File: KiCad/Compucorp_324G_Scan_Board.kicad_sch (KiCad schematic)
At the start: 14 parts, among them J1 BR 16252, J2 Power In, J4 From Keyboard, U1 BR 16252

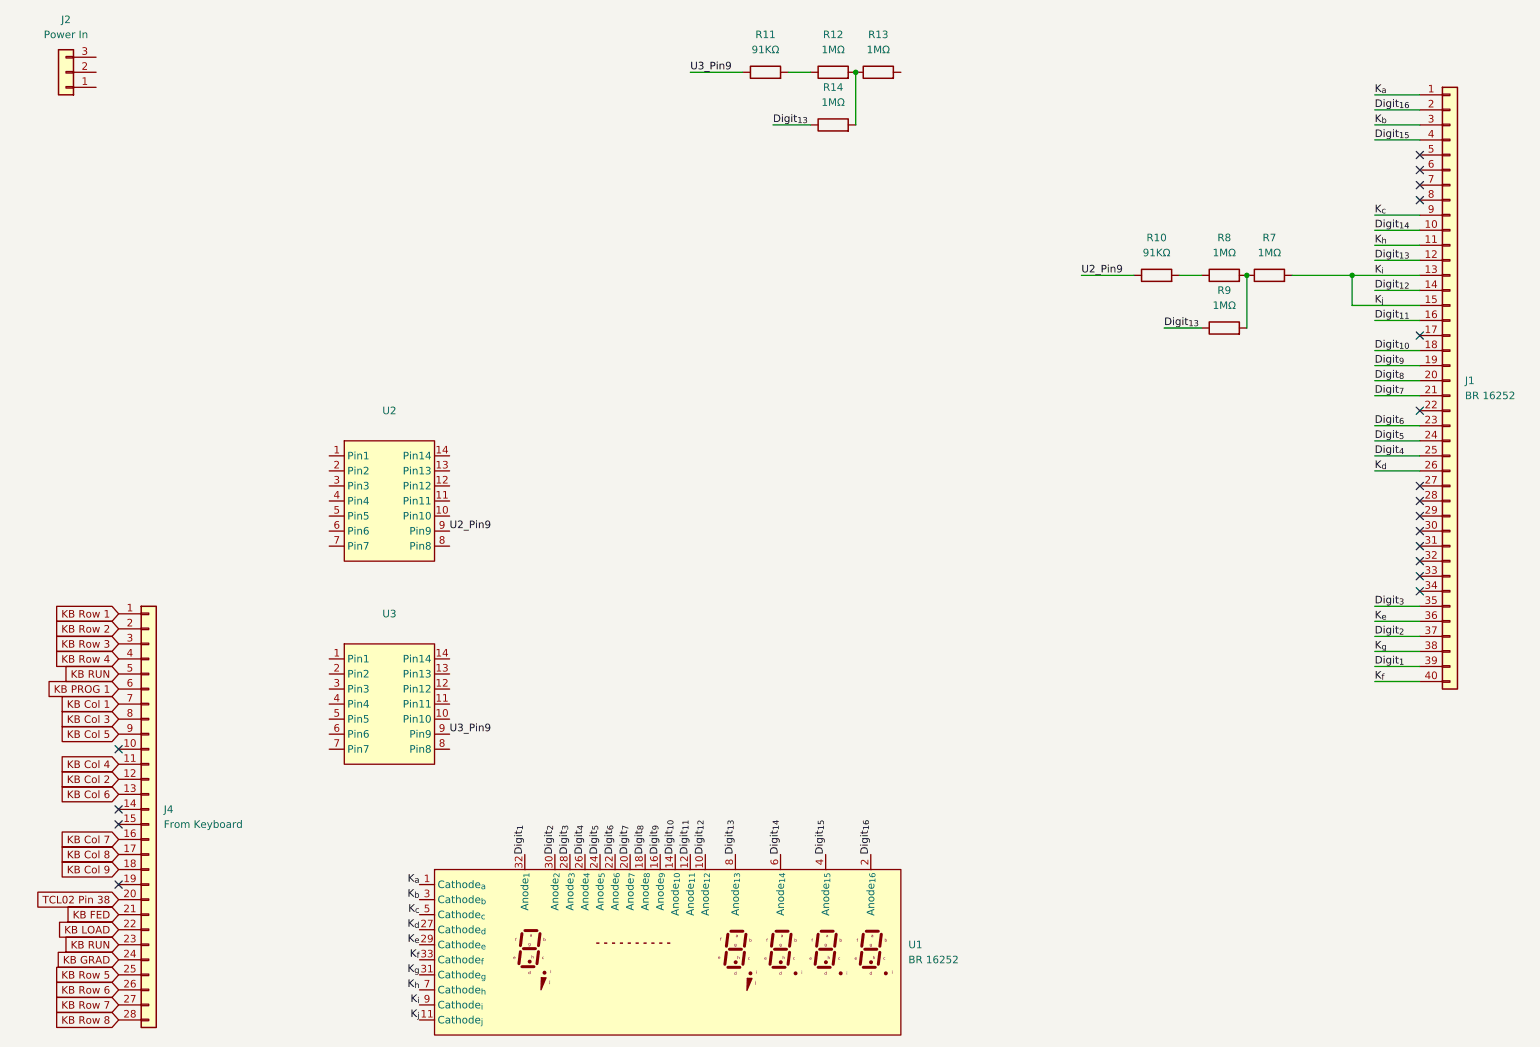
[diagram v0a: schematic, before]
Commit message: Update Compucorp_324G_Scan_Board.kicad_sch
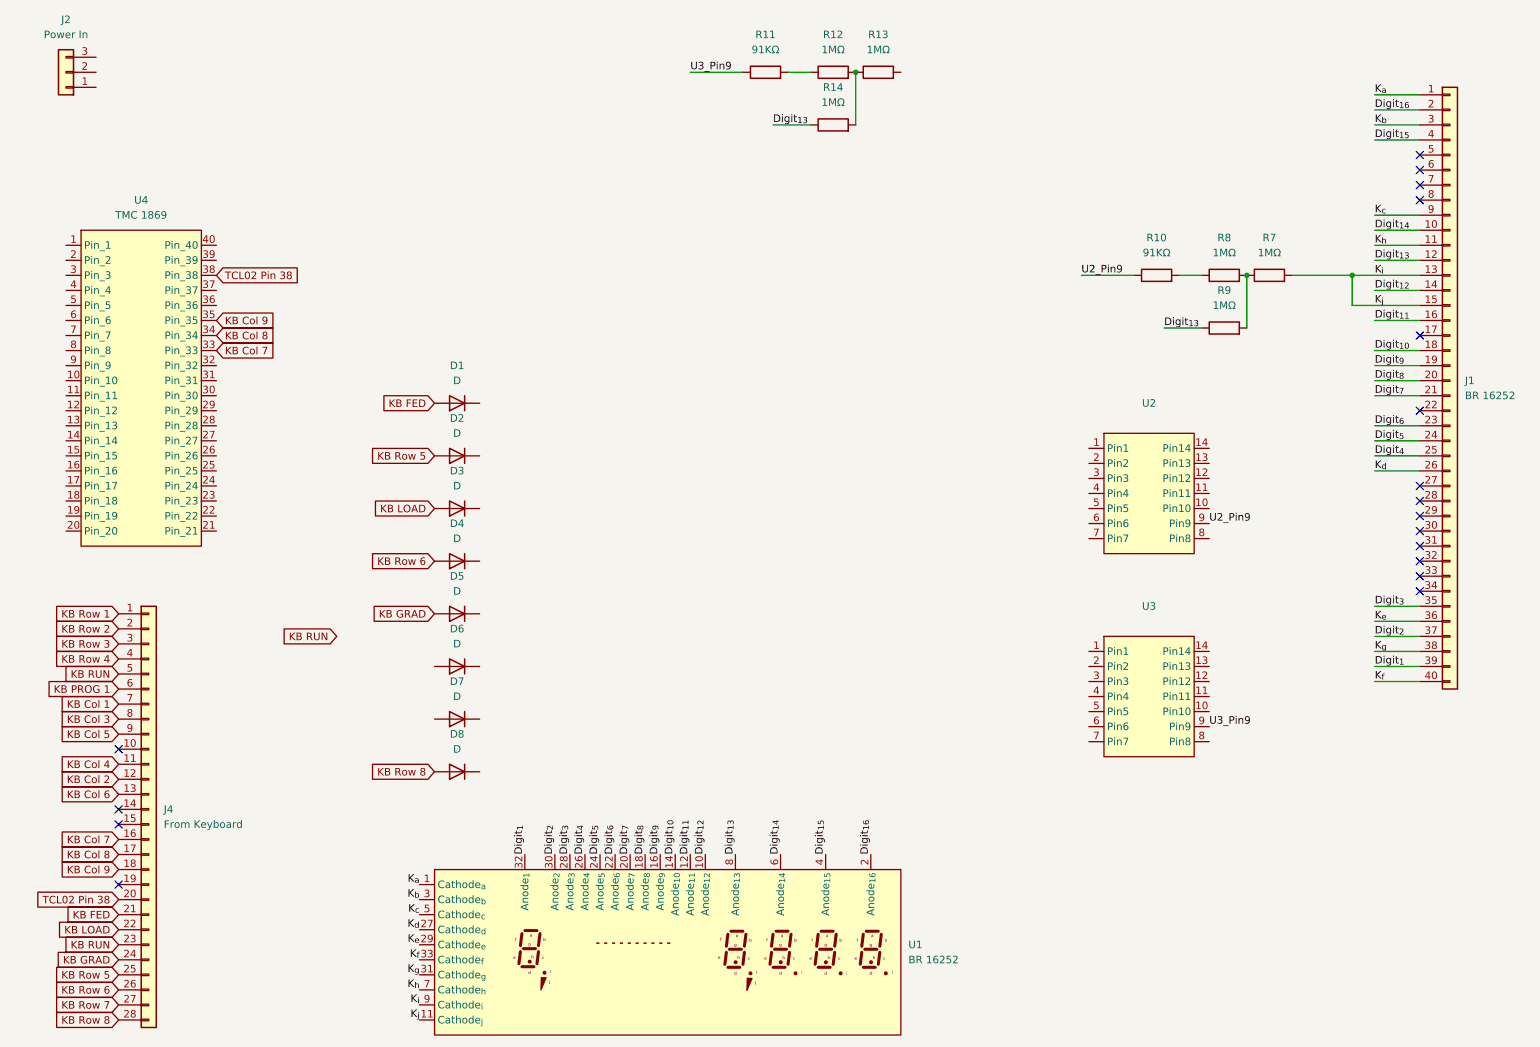
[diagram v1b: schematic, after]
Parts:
- added D1, D2, D3, D4, D5, D6, D7, D8: D, symbol Device:D
- added U4: TMC 1869, symbol Clueless_Engineer:TMC_1869
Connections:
- net KB Col 7: now also U4.33 (Pin_33)
- net KB Col 8: now also U4.34 (Pin_34)
- net KB Col 9: now also U4.35 (Pin_35)
- net KB FED: now also D1.2 (A)
- net KB GRAD: now also D5.2 (A)
- net KB LOAD: now also D3.2 (A)
- net KB Row 5: now also D2.2 (A)
- net KB Row 6: now also D4.2 (A)
- net KB Row 8: now also D8.2 (A)
- net TCL02 Pin 38: now also U4.38 (Pin_38)
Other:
- moved on the sheet: U2, U3
